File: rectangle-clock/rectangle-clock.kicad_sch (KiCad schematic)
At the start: 50 parts, among them J1 Conn_01x07, J2 Power_inlet_vertical, J3 Conn_01x06, J4 Conn_02x03_Odd_Even, SW1 Omron_B3F_SPST, SW2 Omron_B3F_SPST, SW3 Omron_B3F_SPST, SW4 Omron_B3F_SPST, U1 DS1307_DIP-8, U2 L7805, U3 ATmega328-PU, U4 MAX7219, Y1 Crystal_32768Hz, Y2 Crystal_16MHz

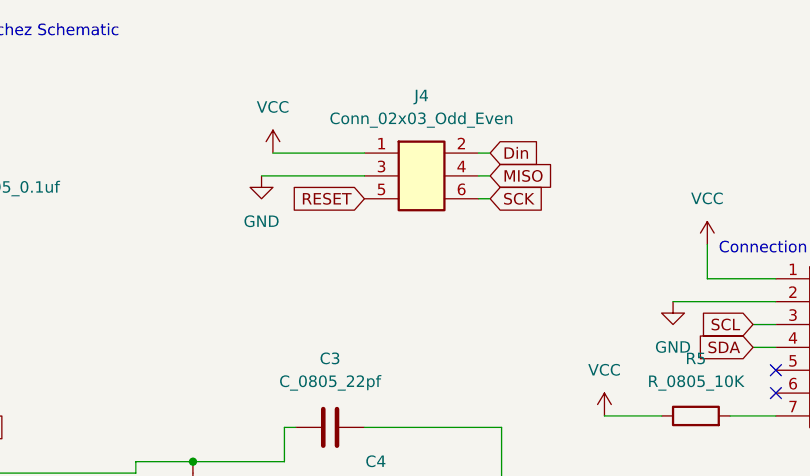
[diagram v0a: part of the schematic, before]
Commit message: Final push? :)
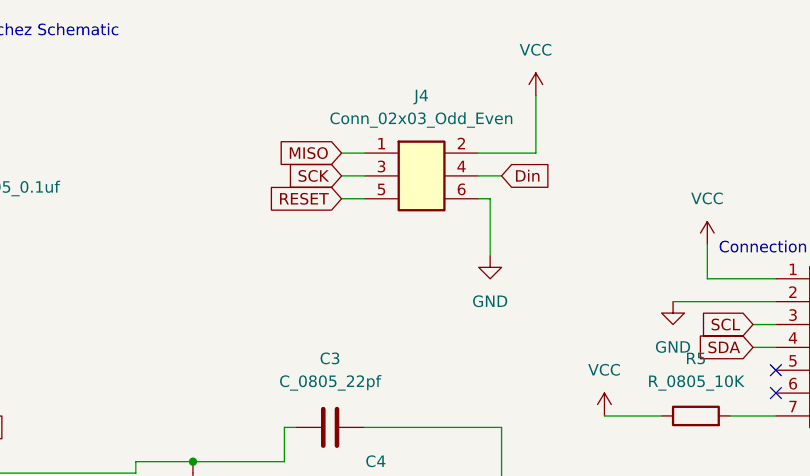
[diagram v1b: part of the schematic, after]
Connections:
- net Din: now also J4.4 (Pin_4); no longer J4.2 (Pin_2)
- net GND: now also J4.6 (Pin_6); no longer J4.3 (Pin_3)
- net MISO: now also J4.1 (Pin_1); no longer J4.4 (Pin_4)
- net SCK: now also J4.3 (Pin_3); no longer J4.6 (Pin_6)
- net VCC: now also J4.2 (Pin_2); no longer J4.1 (Pin_1)
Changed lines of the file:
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@@
+    (stroke (width 0) (type default) (color 0 0 0 0))
+  )
+  (wire (pts (xy 144.78 31.75) (xy 138.43 31.75))
     (stroke (width 0) (type default) (color 0 0 0 0))
   )
@@
     (stroke (width 0) (type default) (color 0 0 0 0))
   )
+  (wire (pts (xy 123.19 36.83) (xy 125.73 36.83))
+    (stroke (width 0) (type default) (color 0 0 0 0))
+  )
   (wire (pts (xy 73.66 90.17) (xy 119.38 90.17))
     (stroke (width 0) (type default) (color 0 0 0 0))
@@
     (stroke (width 0) (type default) (color 0 0 0 0))
   )
-  (wire (pts (xy 139.7 31.75) (xy 138.43 31.75))
-    (stroke (width 0) (type default) (color 0 0 0 0))
-  )
   (wire (pts (xy 125.73 62.23) (xy 140.97 62.23))
     (stroke (width 0) (type default) (color 0 0 0 0))
@@
     (stroke (width 0) (type default) (color 0 0 0 0))
   )
-  (wire (pts (xy 115.57 31.75) (xy 125.73 31.75))
+  (wire (pts (xy 139.7 36.83) (xy 138.43 36.83))
     (stroke (width 0) (type default) (color 0 0 0 0))
   )
@@
     (stroke (width 0) (type default) (color 0 0 0 0))
   )
-  (wire (pts (xy 114.3 34.29) (xy 125.73 34.29))
-    (stroke (width 0) (type default) (color 0 0 0 0))
-  )
   (wire (pts (xy 215.9 73.66) (xy 215.9 77.47))
     (stroke (width 0) (type default) (color 0 0 0 0))
@@
     (stroke (width 0) (type default) (color 0 0 0 0))
   )
+  (wire (pts (xy 140.97 34.29) (xy 138.43 34.29))
+    (stroke (width 0) (type default) (color 0 0 0 0))
+  )
   (wire (pts (xy 76.2 38.1) (xy 76.2 41.91))
     (stroke (width 0) (type default) (color 0 0 0 0))
@@
     (stroke (width 0) (type default) (color 0 0 0 0))
   )
-  (wire (pts (xy 139.7 36.83) (xy 138.43 36.83))
-    (stroke (width 0) (type default) (color 0 0 0 0))
-  )
-  (wire (pts (xy 139.7 34.29) (xy 138.43 34.29))
-    (stroke (width 0) (type default) (color 0 0 0 0))
-  )
   (wire (pts (xy 265.43 113.03) (xy 267.97 113.03))
     (stroke (width 0) (type default) (color 0 0 0 0))
@@
     (stroke (width 0) (type default) (color 0 0 0 0))
   )
+  (wire (pts (xy 123.19 31.75) (xy 125.73 31.75))
+    (stroke (width 0) (type default) (color 0 0 0 0))
+  )
+  (wire (pts (xy 123.19 34.29) (xy 125.73 34.29))
+    (stroke (width 0) (type default) (color 0 0 0 0))
+  )
   (wire (pts (xy 212.09 138.43) (xy 212.09 132.08))
     (stroke (width 0) (type default) (color 0 0 0 0))
@@
     (stroke (width 0) (type default) (color 0 0 0 0))
   )
+  (wire (pts (xy 144.78 25.4) (xy 144.78 31.75))
+    (stroke (width 0) (type default) (color 0 0 0 0))
+  )
   (wire (pts (xy 83.82 168.91) (xy 83.82 181.61))
     (stroke (width 0) (type default) (color 0 0 0 0))
@@
   )
   (wire (pts (xy 58.42 26.67) (xy 58.42 30.48))
+    (stroke (width 0) (type default) (color 0 0 0 0))
+  )
+  (wire (pts (xy 139.7 43.18) (xy 139.7 36.83))
     (stroke (width 0) (type default) (color 0 0 0 0))
   )
@@
     )
   )
-  (global_label "MISO" (shape input) (at 139.7 34.29 0) (fields_autoplaced)
-    (effects (font (size 1.27 1.27)) (justify left))
-    (property "Intersheet References" "${INTERSHEET_REFS}" (id 0) (at 146.7093 34.2106 0)
-      (effects (font (size 1.27 1.27)) (justify left) hide)
+  (global_label "MISO" (shape input) (at 123.19 31.75 180) (fields_autoplaced)
+    (effects (font (size 1.27 1.27)) (justify right))
+    (property "Intersheet References" "${INTERSHEET_REFS}" (id 0) (at 116.1807 31.6706 0)
+      (effects (font (size 1.27 1.27)) (justify right) hide)
     )
   )
@@
     )
   )
-  (global_label "RESET" (shape input) (at 125.73 36.83 180) (fields_autoplaced)
-    (effects (font (size 1.27 1.27)) (justify right))
-    (property "Intersheet References" "${INTERSHEET_REFS}" (id 0) (at 117.5717 36.7506 0)
+  (global_label "RESET" (shape input) (at 123.19 36.83 180) (fields_autoplaced)
+    (effects (font (size 1.27 1.27)) (justify right))
+    (property "Intersheet References" "${INTERSHEET_REFS}" (id 0) (at 115.0317 36.7506 0)
       (effects (font (size 1.27 1.27)) (justify right) hide)
     )
@@
     )
   )
-  (global_label "SCK" (shape input) (at 139.7 36.83 0) (fields_autoplaced)
-    (effects (font (size 1.27 1.27)) (justify left))
-    (property "Intersheet References" "${INTERSHEET_REFS}" (id 0) (at 145.8626 36.7506 0)
-      (effects (font (size 1.27 1.27)) (justify left) hide)
+  (global_label "SCK" (shape input) (at 123.19 34.29 180) (fields_autoplaced)
+    (effects (font (size 1.27 1.27)) (justify right))
+    (property "Intersheet References" "${INTERSHEET_REFS}" (id 0) (at 117.0274 34.2106 0)
+      (effects (font (size 1.27 1.27)) (justify right) hide)
     )
   )
@@
     )
   )
-  (global_label "Din" (shape input) (at 139.7 31.75 0) (fields_autoplaced)
-    (effects (font (size 1.27 1.27)) (justify left))
-    (property "Intersheet References" "${INTERSHEET_REFS}" (id 0) (at 145.1369 31.6706 0)
+  (global_label "Din" (shape input) (at 140.97 34.29 0) (fields_autoplaced)
+    (effects (font (size 1.27 1.27)) (justify left))
+    (property "Intersheet References" "${INTERSHEET_REFS}" (id 0) (at 146.4069 34.2106 0)
       (effects (font (size 1.27 1.27)) (justify left) hide)
     )
@@
     (pin "2")
   )
-  (symbol (lib_id "HPS:VCC") (at 115.57 31.75 0) (unit 1)
-    (in_bom yes) (on_board yes) (fields_autoplaced)
-    (property "Reference" "#PWR0134" (id 0) (at 115.57 35.56 0)
-      (effects (font (size 1.27 1.27)) hide)
-    )
-    (property "Value" "VCC" (id 1) (at 115.57 26.67 0))
-    (property "Footprint" "" (id 2) (at 115.57 31.75 0)
-      (effects (font (size 1.27 1.27)) hide)
-    )
-    (property "Datasheet" "" (id 3) (at 115.57 31.75 0)
+  (symbol (lib_id "HPS:VCC") (at 144.78 25.4 0) (unit 1)
+    (in_bom yes) (on_board yes) (fields_autoplaced)
+    (property "Reference" "#PWR0134" (id 0) (at 144.78 29.21 0)
+      (effects (font (size 1.27 1.27)) hide)
+    )
+    (property "Value" "VCC" (id 1) (at 144.78 20.32 0))
+    (property "Footprint" "" (id 2) (at 144.78 25.4 0)
+      (effects (font (size 1.27 1.27)) hide)
+    )
+    (property "Datasheet" "" (id 3) (at 144.78 25.4 0)
       (effects (font (size 1.27 1.27)) hide)
     )
@@
     (pin "1")
   )
-  (symbol (lib_id "HPS:GND") (at 114.3 34.29 0) (unit 1)
-    (in_bom yes) (on_board yes) (fields_autoplaced)
-    (property "Reference" "#PWR0133" (id 0) (at 114.3 40.64 0)
-      (effects (font (size 1.27 1.27)) hide)
-    )
-    (property "Value" "GND" (id 1) (at 114.3 39.37 0))
-    (property "Footprint" "" (id 2) (at 114.3 34.29 0)
-      (effects (font (size 1.27 1.27)) hide)
-    )
-    (property "Datasheet" "" (id 3) (at 114.3 34.29 0)
-      (effects (font (size 1.27 1.27)) hide)
-    )
+  (symbol (lib_id "HPS:GND") (at 139.7 43.18 0) (unit 1)
+    (in_bom yes) (on_board yes) (fields_autoplaced)
+    (property "Reference" "#PWR0133" (id 0) (at 139.7 49.53 0)
+      (effects (font (size 1.27 1.27)) hide)
+    )
+    (property "Value" "GND" (id 1) (at 139.7 48.26 0))
+    (property "Footprint" "" (id 2) (at 139.7 43.18 0)
+      (effects (font (size 1.27 1.27)) hide)
+    )
+    (property "Datasheet" "" (id 3) (at 139.7 43.18 0)
+      (effects (font (size 1.27 1.27)) hide)
+    )
